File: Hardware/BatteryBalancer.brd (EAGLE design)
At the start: 93.6 x 20.1 mm, 94 parts, among them IC1 OP-AMP, J2 ISP, U1 TAP_POINT, U10 MCP1755, U11 AD7280A, U12 ATMEGA328P_TQFP, U13 CH340C, U2 TAP_POINT, U3 TAP_POINT, U4 TAP_POINT, U5 TAP_POINT, Y1 16MHz

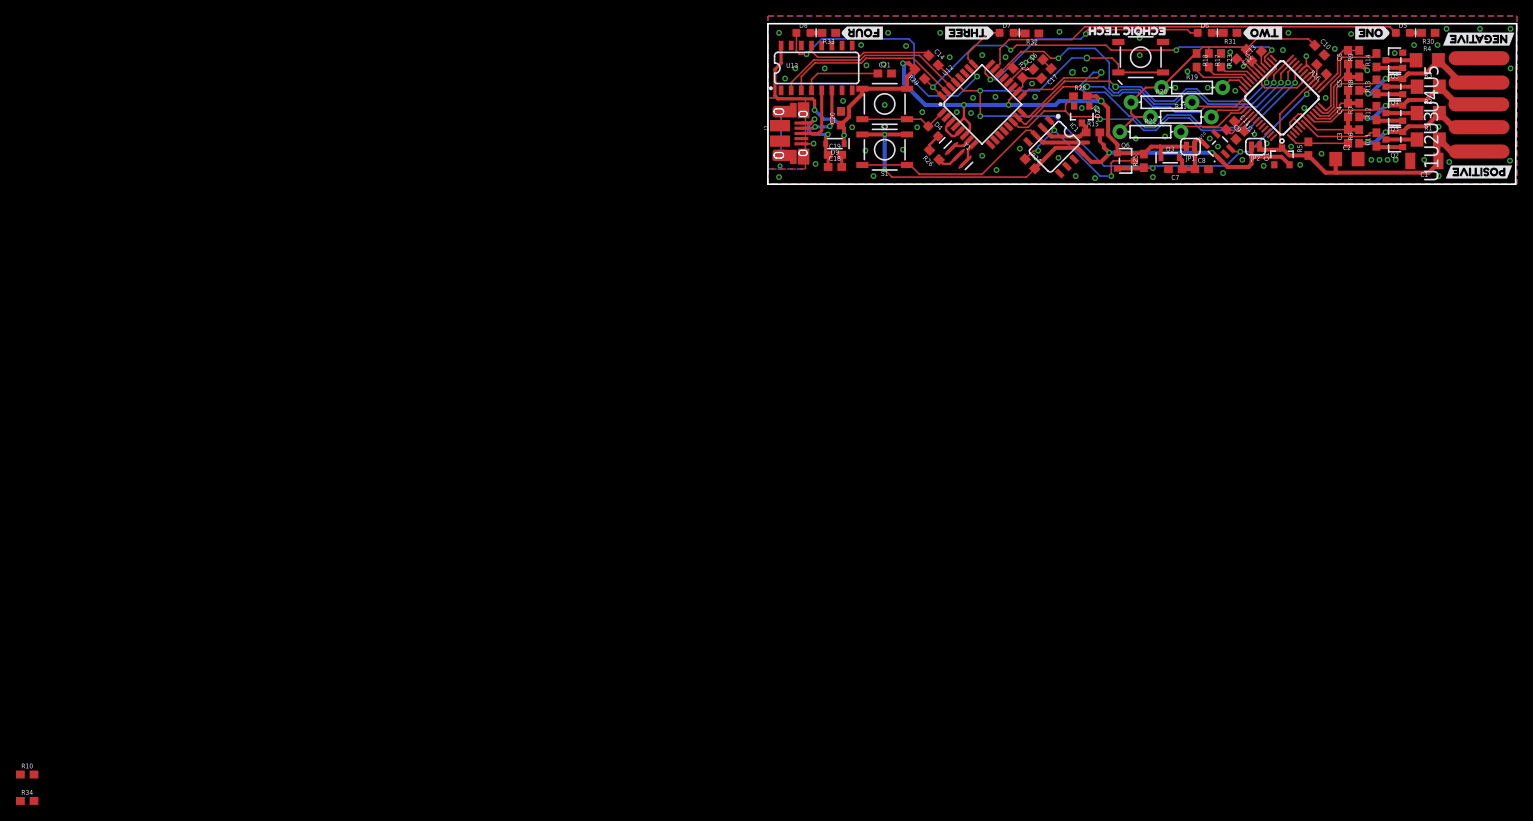
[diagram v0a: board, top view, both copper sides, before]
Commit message: Panelized + cammed
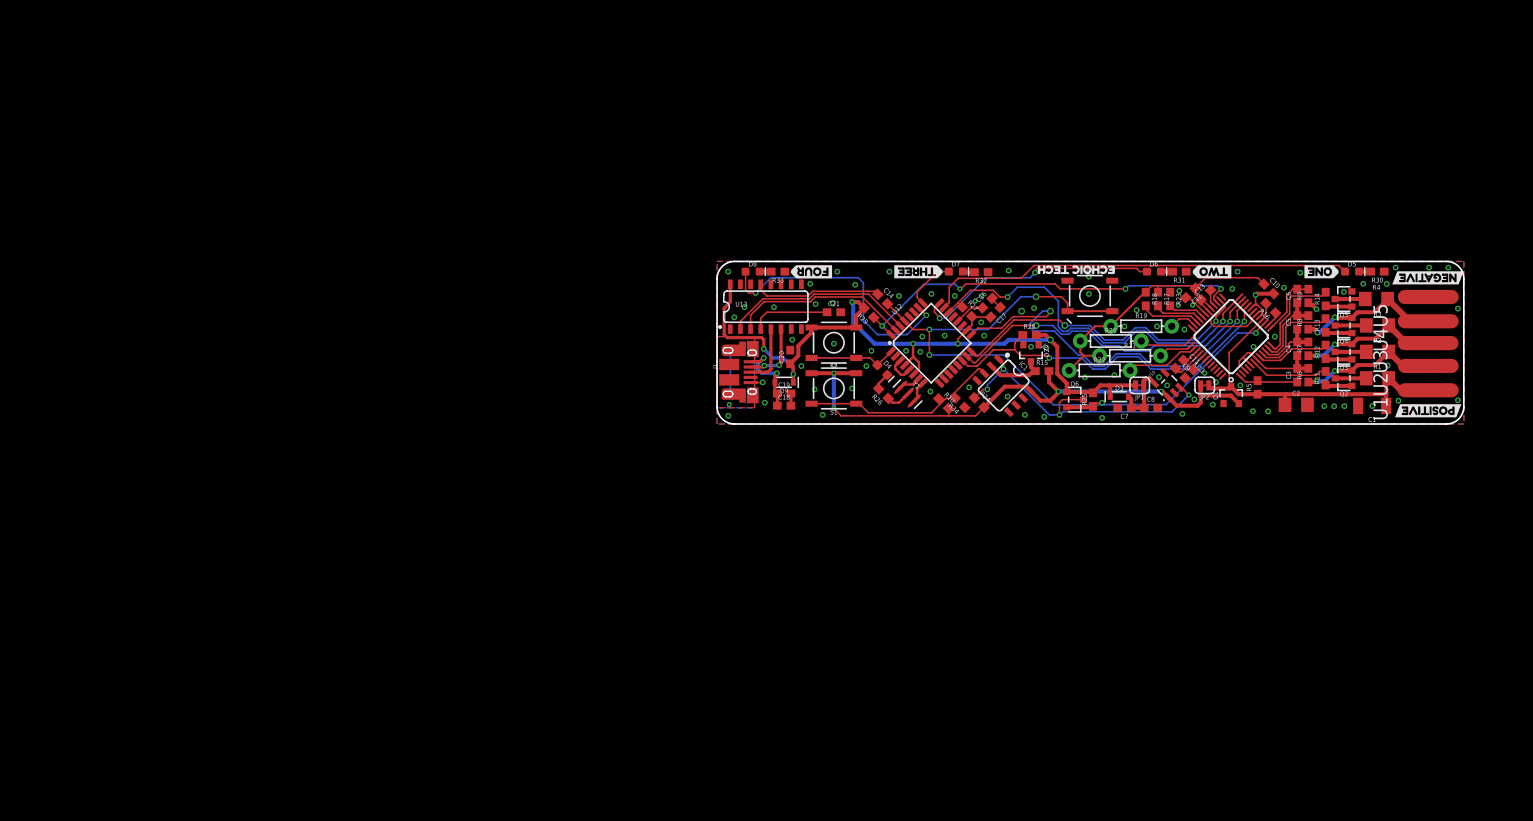
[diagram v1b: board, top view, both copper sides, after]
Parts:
- added U$8: (no value), echoic#JPG:ECHOIC#JPG
- added U$9: (no value), tech#JPG:TECH#JPG
- moved R34 126.8 mm to (30.4, 2.67), turned to 135 degrees
- moved R10 123.6 mm to (28.3, 2.54), turned to 315 degrees
- moved C2 31.4 mm to (72.4, 2.40)
- moved C1 31.3 mm to (81.9, 2.26)
- moved C12 30.5 mm to (59.2, 16.4)
- moved C19 30.5 mm to (8.38, 3.81)
- moved C3 30.5 mm to (72.5, 6.10)
- moved C4 30.5 mm to (72.5, 9.40)
- moved C5 30.5 mm to (72.5, 12.7)
- moved C6 30.5 mm to (72.5, 16.0)
- moved D3 30.5 mm to (50.3, 3.43)
- moved D5 30.5 mm to (79.4, 19.1)
- moved D6 30.5 mm to (54.6, 19.1)
- moved D7 30.5 mm to (29.8, 19.1)
- moved J1 30.5 mm to (4.19, 6.48)
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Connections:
- net RESET renamed !RESET
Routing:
- net CHARGE: track 21.1 -> 39.7 mm, vias 3 -> 4
- net N$40: track 31.6 -> 25.6 mm
- net GND: track 24.5 -> 26.8 mm, vias 89 -> 86
- net V_RAW: track 47.1 -> 45.8 mm
- net !RESET: track 90.1 -> 89.6 mm, vias 5 -> 4
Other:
- board size 93.6 x 20.1 mm -> 93.3 x 20.3 mm
